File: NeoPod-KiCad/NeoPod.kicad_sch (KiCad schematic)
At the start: 62 parts, among them J1 SJ-3523-SMT-TR, J2 USB4500-03-0-A_REVA1, J4 USB4500-03-0-A_REVA1, Q1 CSD25480F3, SW1 SW_SPST, SW2 SW_SPST, SW3 SW_SPST, SW4 SW_SPST, SW5 SW_SPST, U1 ESP32-WROOM-32, U10 SN74CB3Q3257DBQR, U2 PCM5102A, U3 RP2040, U4 CP2102N-Axx-xQFN24, U5 XC6210B332MR, U6 STC4054GR, U7 TFT_320x240, Y2 40MHz-Xtal

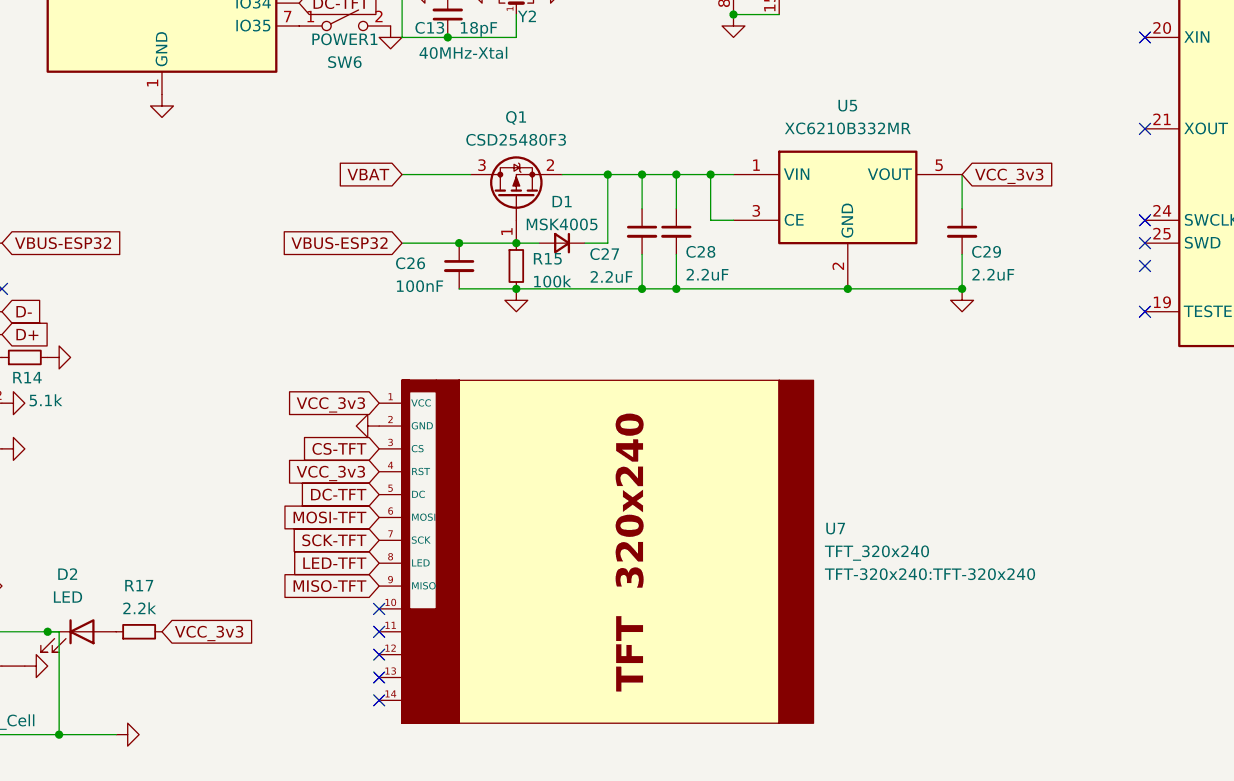
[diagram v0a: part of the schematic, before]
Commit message: finished pcb
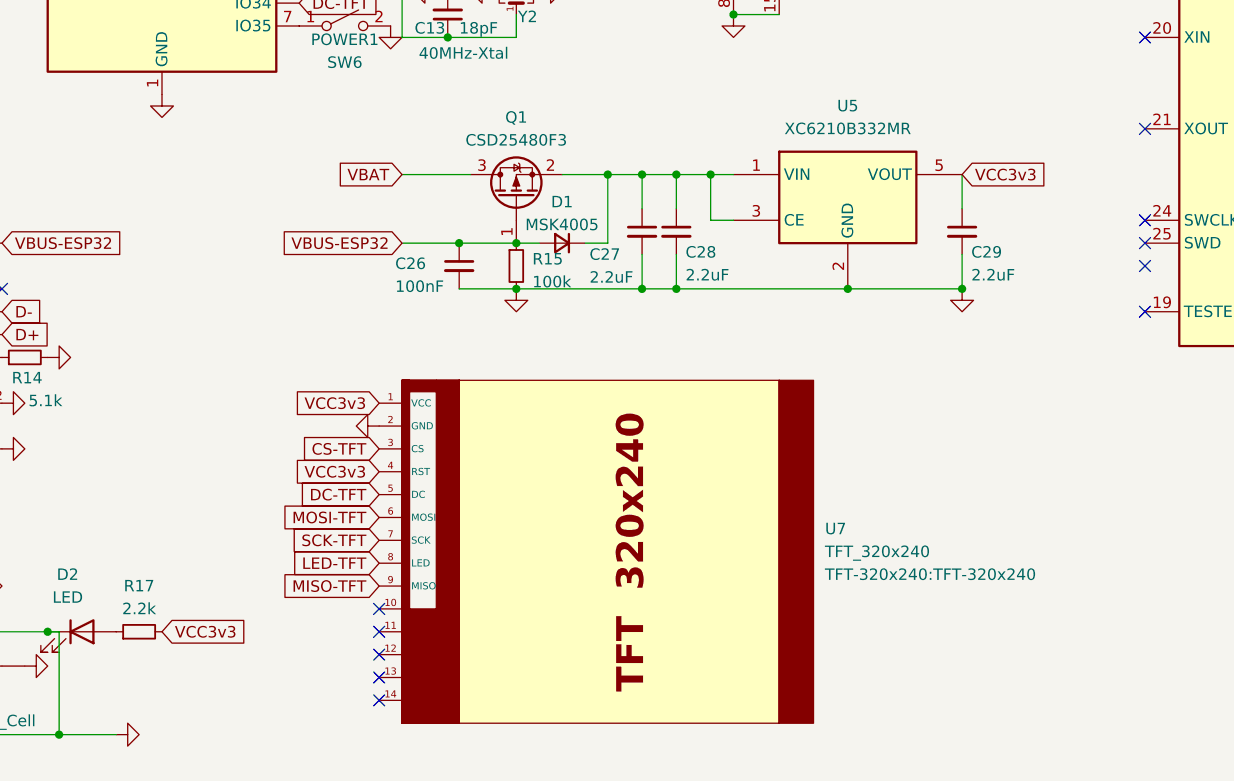
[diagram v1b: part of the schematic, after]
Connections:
- net AGND is gone; now on net GND: C8.2, C9.2, U2.19 (DGND)
- net VCC_3v3 is gone; now on net VCC3v3: C29.1, R17.2, U5.5 (VOUT), U7.1 (VCC), U7.4 (RST)
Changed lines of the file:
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@@
 		)
 	)
+	(global_label "VCC3v3"
+		(shape input)
+		(at 74.93 176.53 0)
+		(fields_autoplaced yes)
+		(effects
+			(font
+				(size 1.27 1.27)
+			)
+			(justify left)
+		)
+		(property "Intersheetrefs" "${INTERSHEET_REFS}"
+			(at 84.9304 176.53 0)
+			(effects
+				(font
+					(size 1.27 1.27)
+				)
+				(justify left)
+				(hide yes)
+			)
+		)
+	)
 	(global_label "VCC3v3a"
 		(shape input)
@@
 		)
 	)
-	(global_label "VCC_3v3"
-		(shape input)
-		(at 163.83 125.73 0)
-		(fields_autoplaced yes)
-		(effects
-			(font
-				(size 1.27 1.27)
-			)
-			(justify left)
-		)
-		(property "Intersheetrefs" "${INTERSHEET_REFS}"
-			(at 174.798 125.73 0)
-			(effects
-				(font
-					(size 1.27 1.27)
-				)
-				(justify left)
-				(hide yes)
-			)
-		)
-	)
 	(global_label "VBUS-ESP32"
 		(shape input)
@@
 		)
 	)
+	(global_label "VCC3v3"
+		(shape input)
+		(at 99.06 158.75 180)
+		(fields_autoplaced yes)
+		(effects
+			(font
+				(size 1.27 1.27)
+			)
+			(justify right)
+		)
+		(property "Intersheetrefs" "${INTERSHEET_REFS}"
+			(at 89.0596 158.75 0)
+			(effects
+				(font
+					(size 1.27 1.27)
+				)
+				(justify right)
+				(hide yes)
+			)
+		)
+	)
 	(global_label "VBAT"
 		(shape input)
@@
 		)
 	)
+	(global_label "VCC3v3"
+		(shape input)
+		(at 99.06 151.13 180)
+		(fields_autoplaced yes)
+		(effects
+			(font
+				(size 1.27 1.27)
+			)
+			(justify right)
+		)
+		(property "Intersheetrefs" "${INTERSHEET_REFS}"
+			(at 89.0596 151.13 0)
+			(effects
+				(font
+					(size 1.27 1.27)
+				)
+				(justify right)
+				(hide yes)
+			)
+		)
+	)
 	(global_label "SW2"
 		(shape input)
@@
 		)
 	)
-	(global_label "VCC_3v3"
-		(shape input)
-		(at 74.93 176.53 0)
-		(fields_autoplaced yes)
-		(effects
-			(font
-				(size 1.27 1.27)
-			)
-			(justify left)
-		)
-		(property "Intersheetrefs" "${INTERSHEET_REFS}"
-			(at 85.898 176.53 0)
-			(effects
-				(font
-					(size 1.27 1.27)
-				)
-				(justify left)
-				(hide yes)
-			)
-		)
-	)
 	(global_label "DP"
 		(shape input)
@@
 		)
 	)
-	(global_label "VCC_3v3"
-		(shape input)
-		(at 99.06 158.75 180)
-		(fields_autoplaced yes)
-		(effects
-			(font
-				(size 1.27 1.27)
-			)
-			(justify right)
-		)
-		(property "Intersheetrefs" "${INTERSHEET_REFS}"
-			(at 88.092 158.75 0)
-			(effects
-				(font
-					(size 1.27 1.27)
-				)
-				(justify right)
-				(hide yes)
-			)
-		)
-	)
 	(global_label "MOSI-SD"
 		(shape input)
@@
 		)
 	)
+	(global_label "VCC3v3"
+		(shape input)
+		(at 163.83 125.73 0)
+		(fields_autoplaced yes)
+		(effects
+			(font
+				(size 1.27 1.27)
+			)
+			(justify left)
+		)
+		(property "Intersheetrefs" "${INTERSHEET_REFS}"
+			(at 173.8304 125.73 0)
+			(effects
+				(font
+					(size 1.27 1.27)
+				)
+				(justify left)
+				(hide yes)
+			)
+		)
+	)
 	(global_label "VBUS-ESP32"
 		(shape input)
@@
 		)
 	)
-	(global_label "VCC_3v3"
-		(shape input)
-		(at 99.06 151.13 180)
-		(fields_autoplaced yes)
-		(effects
-			(font
-				(size 1.27 1.27)
-			)
-			(justify right)
-		)
-		(property "Intersheetrefs" "${INTERSHEET_REFS}"
-			(at 88.092 151.13 0)
-			(effects
-				(font
-					(size 1.27 1.27)
-				)
-				(justify right)
-				(hide yes)
-			)
-		)
-	)
 	(global_label "VCC3v3"
 		(shape input)
@@
 			)
 		)
-		(property "Value" "AGND"
+		(property "Value" "GND"
 			(at 137.16 26.67 0)
 			(effects
@@
 			)
 		)
-		(property "Value" "AGND"
+		(property "Value" "GND"
 			(at 124.46 71.12 0)
 			(effects
